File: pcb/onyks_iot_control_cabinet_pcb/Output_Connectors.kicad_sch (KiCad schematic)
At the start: 2 parts, among them J5 Conn_02x09_Odd_Even, J6 Conn_01x06_Socket

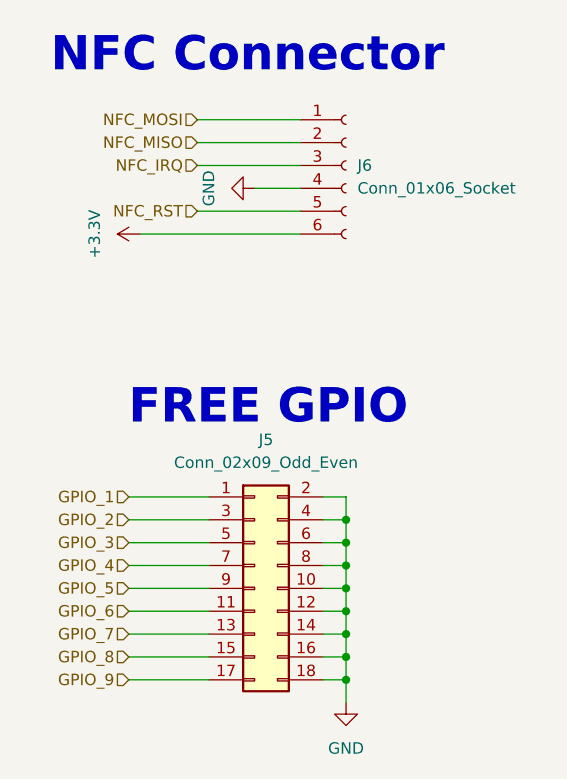
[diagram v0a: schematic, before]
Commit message: Quick Fixes
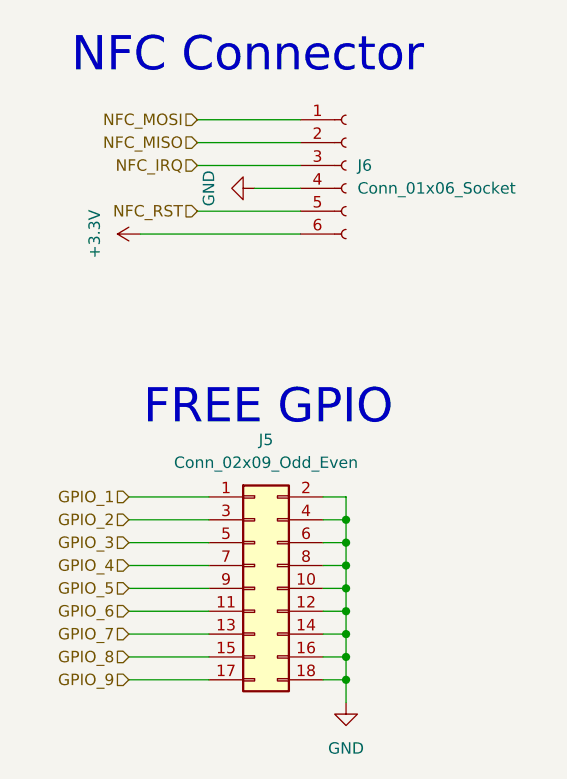
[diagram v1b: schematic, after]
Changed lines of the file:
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@@
 			(font
 				(size 3.81 3.81)
-				(thickness 0.762)
-				(bold yes)
+				(thickness 0.4763)
 			)
 		)
@@
 			(font
 				(size 3.81 3.81)
-				(thickness 0.762)
-				(bold yes)
+				(thickness 0.4763)
 			)
 		)
